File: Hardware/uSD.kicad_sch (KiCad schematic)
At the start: 2 parts, among them J12 MSD-4-A

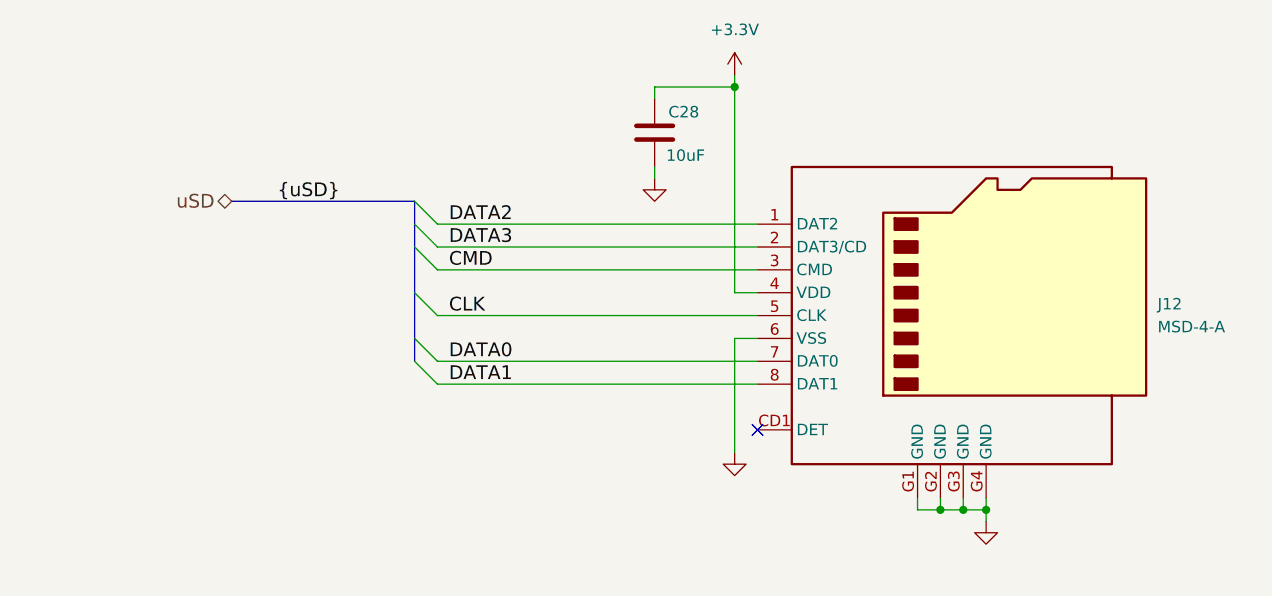
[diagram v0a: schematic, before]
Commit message: S31 fully connected
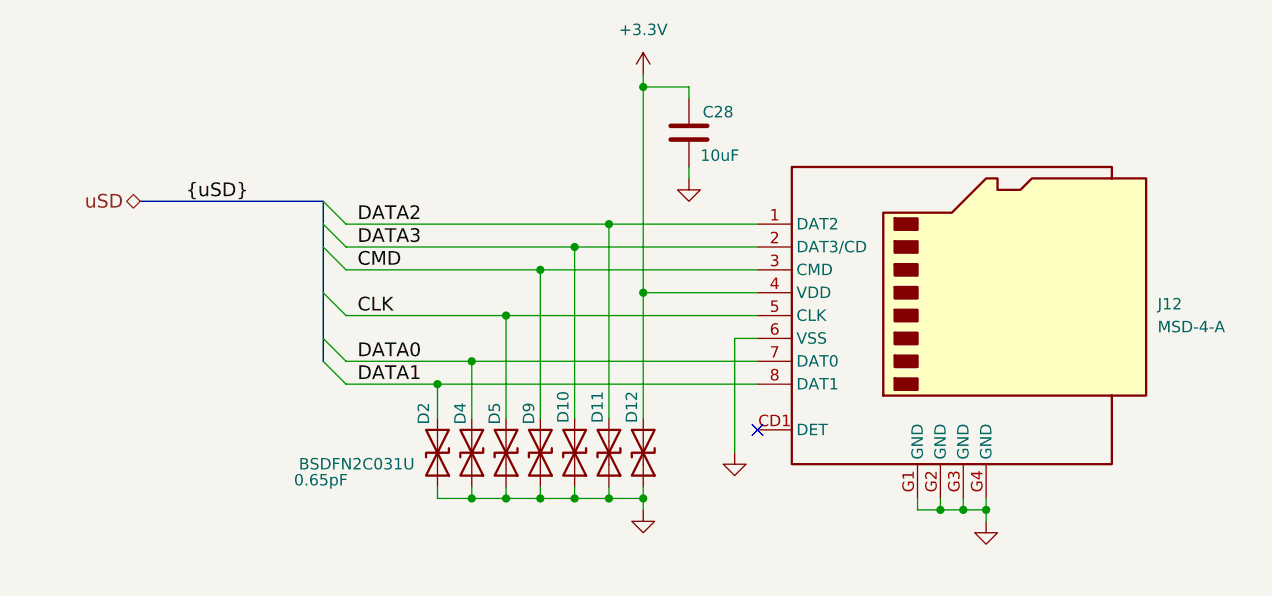
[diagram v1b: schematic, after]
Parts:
- added D10, D11, D12, D2, D4, D5, D9: BSDFN2C031U, PCM_JLCPCB:D_DFN1006-2L, symbol YV-library:TVS-BSDFN2C031U
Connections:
- net +3.3V: now also D12.2 (A2)
- net CLK: now also D5.2 (A2)
- net CMD: now also D9.2 (A2)
- net DATA0: now also D4.2 (A2)
- net DATA1: now also D2.2 (A2)
- net DATA2: now also D11.2 (A2)
- net DATA3: now also D10.2 (A2)
- net GND: now also D10.1 (A1), D11.1 (A1), D12.1 (A1), D2.1 (A1), D4.1 (A1), D5.1 (A1), D9.1 (A1)
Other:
- moved on the sheet: C28

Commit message: Schematic Done
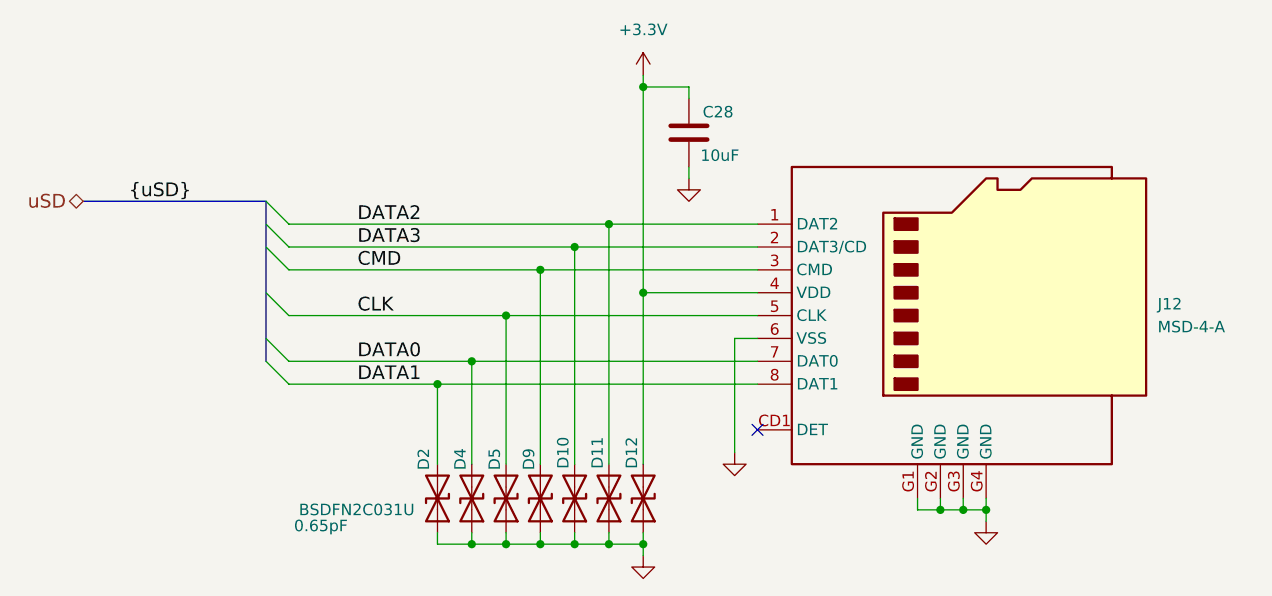
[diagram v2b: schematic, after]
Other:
- company: (none) -> Motion Composites
- title: (none) -> Strain Gauge Data Logger
- moved on the sheet: D10, D11, D12, D2, D4, D5, D9
